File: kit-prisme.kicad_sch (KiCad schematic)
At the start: 95 parts, among them J1 Conn_01x02, J10 Conn_01x03, J11 Conn_01x04, J12 Conn_01x04, J13 Conn_01x04, J14 Conn_01x04, J15 Conn_01x04, J16 Conn_01x04, J17 Conn_01x04, J18 Conn_01x04, J19 Conn_01x04, J2 Conn_01x16, J20 Conn_01x04, J21 Conn_01x04, J22 Conn_01x04, J23 Conn_01x04, J24 Conn_01x04, J25 Conn_01x04, J26 Conn_01x04, J3 Conn_01x16, J4 Conn_01x16, J5 Conn_01x02, J6 Conn_01x02, J7 Conn_01x04, J8 Conn_01x04, J9 Conn_01x04, Q1 2N7000, Q10 2N7000, Q11 2N7000, Q2 2N7000, Q3 2N7000, Q4 2N7000, Q5 2N7000, Q6 2N7000, Q7 2N7000, Q8 2N7000, Q9 2N7000

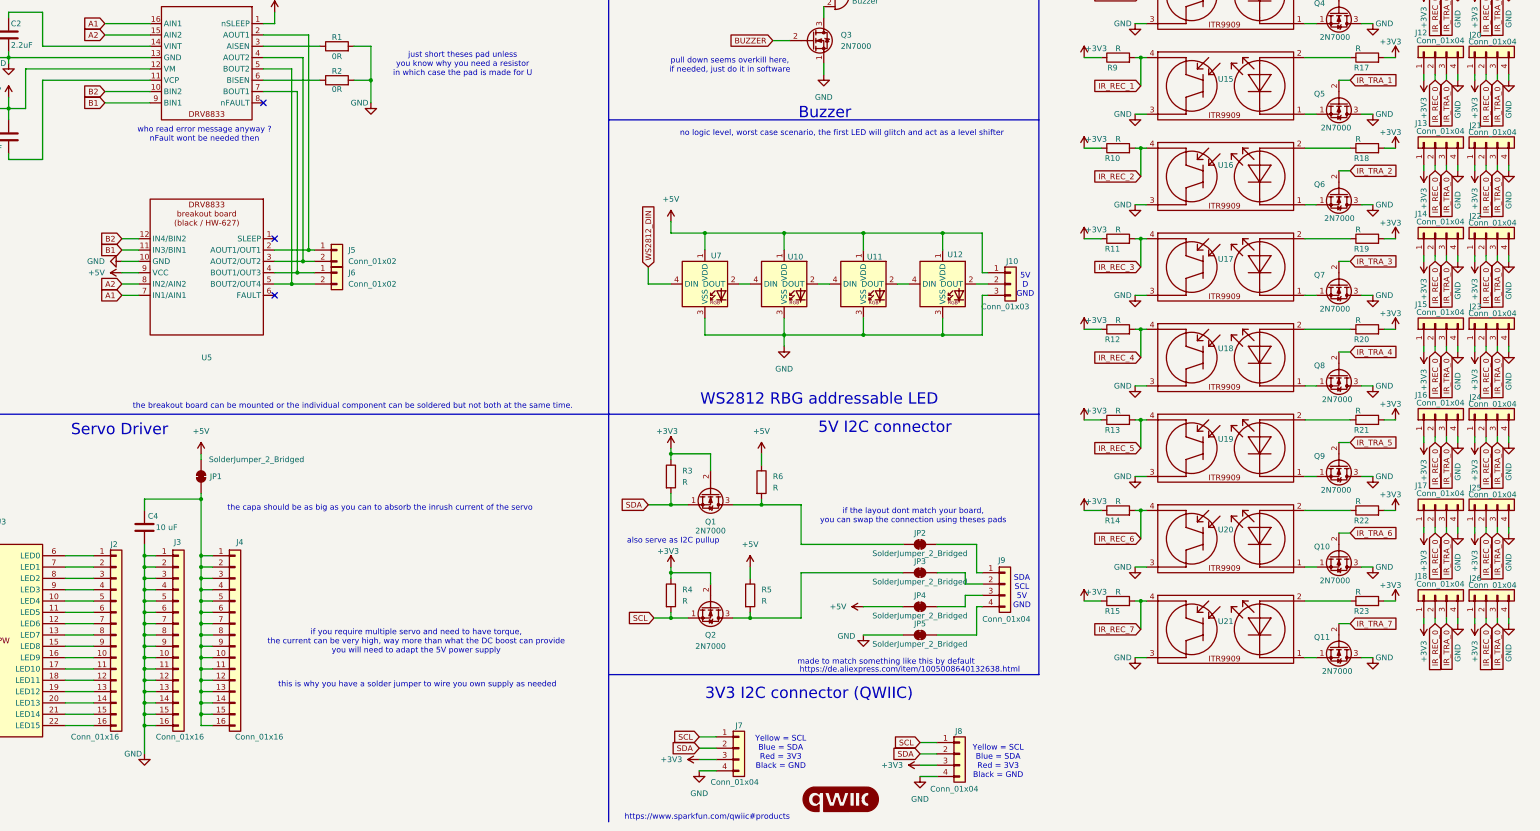
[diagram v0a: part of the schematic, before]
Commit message: looking for a good PCB layout
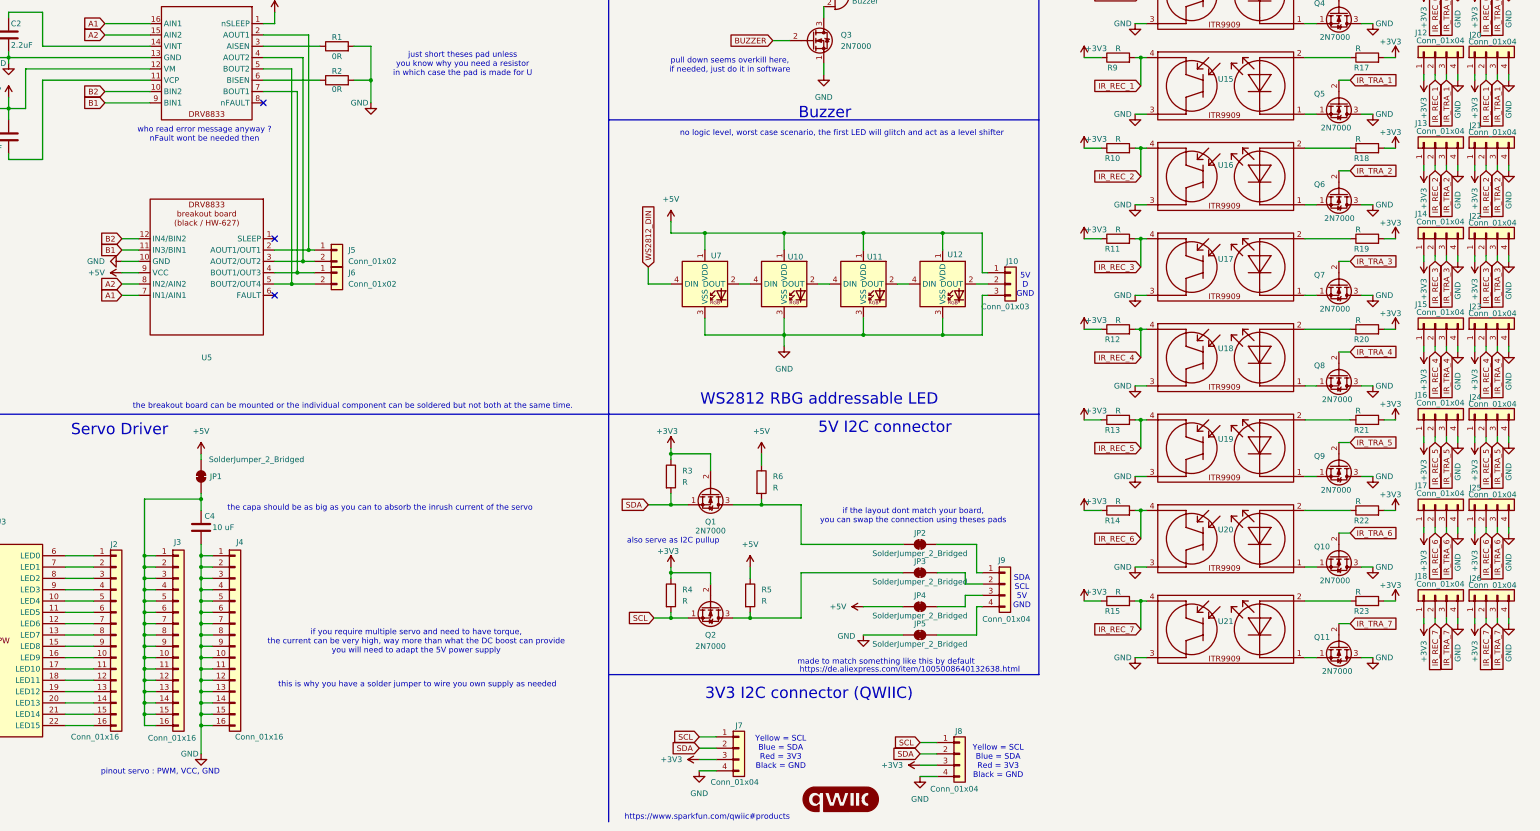
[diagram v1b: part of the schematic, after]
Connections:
- net GND: now also J4.1 (Pin_1), J4.10 (Pin_10), J4.11 (Pin_11), J4.12 (Pin_12), J4.13 (Pin_13), J4.14 (Pin_14), J4.15 (Pin_15), J4.16 (Pin_16), J4.2 (Pin_2), J4.3 (Pin_3), J4.4 (Pin_4), J4.5 (Pin_5), J4.6 (Pin_6), J4.7 (Pin_7), J4.8 (Pin_8), J4.9 (Pin_9); no longer J3.1 (Pin_1), J3.10 (Pin_10), J3.11 (Pin_11), J3.12 (Pin_12), J3.13 (Pin_13), J3.14 (Pin_14), J3.15 (Pin_15), J3.16 (Pin_16), J3.2 (Pin_2), J3.3 (Pin_3), J3.4 (Pin_4), J3.5 (Pin_5), J3.6 (Pin_6), J3.7 (Pin_7), J3.8 (Pin_8), J3.9 (Pin_9)
- net IR_REC_0: no longer J12.2 (Pin_2), J13.2 (Pin_2), J14.2 (Pin_2), J15.2 (Pin_2), J16.2 (Pin_2), J17.2 (Pin_2), J18.2 (Pin_2), J20.2 (Pin_2), J21.2 (Pin_2), J22.2 (Pin_2), J23.2 (Pin_2), J24.2 (Pin_2), J25.2 (Pin_2), J26.2 (Pin_2)
- net IR_REC_1: now also J12.2 (Pin_2), J20.2 (Pin_2)
- net IR_REC_2: now also J13.2 (Pin_2), J21.2 (Pin_2)
- net IR_REC_3: now also J14.2 (Pin_2), J22.2 (Pin_2)
- net IR_REC_4: now also J15.2 (Pin_2), J23.2 (Pin_2)
- net IR_REC_5: now also J16.2 (Pin_2), J24.2 (Pin_2)
- net IR_REC_6: now also J17.2 (Pin_2), J25.2 (Pin_2)
- net IR_REC_7: now also J18.2 (Pin_2), J26.2 (Pin_2)
- net IR_TRA_0: no longer J12.3 (Pin_3), J13.3 (Pin_3), J14.3 (Pin_3), J15.3 (Pin_3), J16.3 (Pin_3), J17.3 (Pin_3), J18.3 (Pin_3), J20.3 (Pin_3), J21.3 (Pin_3), J22.3 (Pin_3), J23.3 (Pin_3), J24.3 (Pin_3), J25.3 (Pin_3), J26.3 (Pin_3)
- net IR_TRA_1: now also J12.3 (Pin_3), J20.3 (Pin_3)
- net IR_TRA_2: now also J13.3 (Pin_3), J21.3 (Pin_3)
- net IR_TRA_3: now also J14.3 (Pin_3), J22.3 (Pin_3)
- net IR_TRA_4: now also J15.3 (Pin_3), J23.3 (Pin_3)
- net IR_TRA_5: now also J16.3 (Pin_3), J24.3 (Pin_3)
- net IR_TRA_6: now also J17.3 (Pin_3), J25.3 (Pin_3)
- net IR_TRA_7: now also J18.3 (Pin_3), J26.3 (Pin_3)
- new net: C4.1, J3.1 (Pin_1), J3.10 (Pin_10), J3.11 (Pin_11), J3.12 (Pin_12), J3.13 (Pin_13), J3.14 (Pin_14), J3.15 (Pin_15), J3.16 (Pin_16), J3.2 (Pin_2), J3.3 (Pin_3), J3.4 (Pin_4), J3.5 (Pin_5), J3.6 (Pin_6), J3.7 (Pin_7), J3.8 (Pin_8), J3.9 (Pin_9), JP1.2 (B)
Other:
- note added: "pinout servo : PWM, VCC, GND"
- moved on the sheet: C4
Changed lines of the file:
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@@
 		)
 	)
+	(text "pinout servo : PWM, VCC, GND\n"
+		(exclude_from_sim no)
+		(at 102.616 273.304 0)
+		(effects
+			(font
+				(size 1.27 1.27)
+			)
+		)
+	)
 	(text "also serve as I2C pullup"
 		(exclude_from_sim no)
@@
 	)
 	(junction
+		(at 111.76 224.79)
+		(diameter 0)
+		(color 0 0 0 0)
+	)
+	(junction
 		(at 99.06 252.73)
 		(diameter 0)
@@
 	)
 	(junction
+		(at 111.76 212.09)
+		(diameter 0)
+		(color 0 0 0 0)
+	)
+	(junction
 		(at 260.35 152.4)
 		(diameter 0)
@@
 	)
 	(junction
-		(at 111.76 212.09)
+		(at 111.76 262.89)
 		(diameter 0)
 		(color 0 0 0 0)
@@
 	)
 	(junction
-		(at 99.06 262.89)
-		(diameter 0)
-		(color 0 0 0 0)
-	)
-	(junction
 		(at 38.1 57.15)
 		(diameter 0)
@@
 	)
 	(junction
-		(at 111.76 224.79)
-		(diameter 0)
-		(color 0 0 0 0)
-	)
-	(junction
 		(at 99.06 242.57)
 		(diameter 0)
@@
 	(wire
 		(pts
+			(xy 111.76 222.25) (xy 111.76 224.79)
+		)
+		(stroke
+			(width 0)
+			(type default)
+		)
+	)
+	(wire
+		(pts
 			(xy 242.57 171.45) (xy 242.57 175.26)
 		)
@@
 	(wire
 		(pts
-			(xy 99.06 222.25) (xy 99.06 224.79)
-		)
-		(stroke
-			(width 0)
-			(type default)
-		)
-	)
-	(wire
-		(pts
 			(xy 278.13 175.26) (xy 287.02 175.26)
 		)
@@
 	(wire
 		(pts
-			(xy 111.76 212.09) (xy 111.76 224.79)
-		)
-		(stroke
-			(width 0)
-			(type default)
-		)
-	)
-	(wire
-		(pts
 			(xy 322.58 133.35) (xy 322.58 139.7)
 		)
@@
 	(wire
 		(pts
+			(xy 111.76 212.09) (xy 111.76 214.63)
+		)
+		(stroke
+			(width 0)
+			(type default)
+		)
+	)
+	(wire
+		(pts
 			(xy 241.3 25.4) (xy 243.84 25.4)
 		)
@@
 	(wire
 		(pts
-			(xy 99.06 214.63) (xy 99.06 212.09)
+			(xy 99.06 212.09) (xy 99.06 224.79)
 		)
 		(stroke
@@
 	(wire
 		(pts
+			(xy 111.76 262.89) (xy 111.76 269.24)
+		)
+		(stroke
+			(width 0)
+			(type default)
+		)
+	)
+	(wire
+		(pts
 			(xy 326.39 62.23) (xy 326.39 63.5)
 		)
@@
 	(wire
 		(pts
-			(xy 99.06 262.89) (xy 99.06 269.24)
-		)
-		(stroke
-			(width 0)
-			(type default)
-		)
-	)
-	(wire
-		(pts
 			(xy 45.72 252.73) (xy 43.18 252.73)
 		)
@@
 		)
 	)
-	(global_label "IR_REC_0"
+	(global_label "IR_REC_1"
 		(shape input)
 		(at 400.05 118.11 270)
@@
 		)
 	)
-	(global_label "IR_REC_0"
+	(global_label "IR_REC_1"
 		(shape input)
 		(at 388.62 118.11 270)
@@
 		)
 	)
-	(global_label "IR_TRA_0"
+	(global_label "IR_TRA_5"
 		(shape input)
 		(at 402.59 199.39 270)
@@
 		)
 	)
-	(global_label "IR_TRA_0"
+	(global_label "IR_TRA_7"
 		(shape input)
 		(at 391.16 240.03 270)
@@
 		)
 	)
-	(global_label "IR_REC_0"
+	(global_label "IR_REC_6"
 		(shape input)
 		(at 388.62 219.71 270)
@@
 		)
 	)
-	(global_label "IR_TRA_0"
+	(global_label "IR_TRA_1"
 		(shape input)
 		(at 402.59 118.11 270)
@@
 		)
 	)
-	(global_label "IR_REC_0"
+	(global_label "IR_REC_7"
 		(shape input)
 		(at 400.05 240.03 270)
@@
 		)
 	)
-	(global_label "IR_TRA_0"
+	(global_label "IR_TRA_3"
 		(shape input)
 		(at 402.59 158.75 270)
@@
 		)
 	)
-	(global_label "IR_TRA_0"
+	(global_label "IR_TRA_4"
 		(shape input)
 		(at 391.16 179.07 270)
@@
 		)
 	)
-	(global_label "IR_REC_0"
+	(global_label "IR_REC_4"
 		(shape input)
 		(at 388.62 179.07 270)
@@
 		)
 	)
-	(global_label "IR_TRA_0"
+	(global_label "IR_TRA_6"
 		(shape input)
 		(at 402.59 219.71 270)
@@
 		)
 	)
-	(global_label "IR_TRA_0"
+	(global_label "IR_TRA_2"
 		(shape input)
 		(at 391.16 138.43 270)
@@
 		)
 	)
-	(global_label "IR_TRA_0"
+	(global_label "IR_TRA_3"
 		(shape input)
 		(at 391.16 158.75 270)
@@
 		)
 	)
-	(global_label "IR_REC_0"
+	(global_label "IR_REC_2"
 		(shape input)
 		(at 400.05 138.43 270)
@@
 		)
 	)
-	(global_label "IR_TRA_0"
+	(global_label "IR_TRA_2"
 		(shape input)
 		(at 402.59 138.43 270)
@@
 		)
 	)
-	(global_label "IR_REC_0"
+	(global_label "IR_REC_4"
 		(shape input)
 		(at 400.05 179.07 270)
@@
 		)
 	)
-	(global_label "IR_REC_0"
+	(global_label "IR_REC_5"
 		(shape input)
 		(at 400.05 199.39 270)
@@
 		)
 	)
-	(global_label "IR_TRA_0"
+	(global_label "IR_TRA_5"
 		(shape input)
 		(at 391.16 199.39 270)
@@
 		)
 	)
-	(global_label "IR_REC_0"
+	(global_label "IR_REC_3"
 		(shape input)
 		(at 388.62 158.75 270)
@@
 		)
 	)
-	(global_label "IR_REC_0"
+	(global_label "IR_REC_2"
 		(shape input)
 		(at 388.62 138.43 270)
@@
 		)
 	)
-	(global_label "IR_REC_0"
+	(global_label "IR_REC_5"
 		(shape input)
 		(at 388.62 199.39 270)
@@
 		)
 	)
-	(global_label "IR_REC_0"
+	(global_label "IR_REC_6"
 		(shape input)
 		(at 400.05 219.71 270)
@@
 		)
 	)
-	(global_label "IR_TRA_0"
+	(global_label "IR_TRA_1"
 		(shape input)
 		(at 391.16 118.11 270)
@@
 		)
 	)
-	(global_label "IR_TRA_0"
+	(global_label "IR_TRA_7"
 		(shape input)
 		(at 402.59 240.03 270)
@@
 		)
 	)
-	(global_label "IR_REC_0"
+	(global_label "IR_REC_7"
 		(shape input)
 		(at 388.62 240.03 270)
@@
 		)
 	)
-	(global_label "IR_TRA_0"
+	(global_label "IR_TRA_6"
 		(shape input)
 		(at 391.16 219.71 270)
@@
 		)
 	)
-	(global_label "IR_TRA_0"
+	(global_label "IR_TRA_4"
 		(shape input)
 		(at 402.59 179.07 270)
@@
 		)
 	)
-	(global_label "IR_REC_0"
+	(global_label "IR_REC_3"
 		(shape input)
 		(at 400.05 158.75 270)
@@
 	(symbol
 		(lib_id "power:GND")
-		(at 99.06 269.24 0)
+		(at 111.76 269.24 0)
 		(unit 1)
 		(exclude_from_sim no)
@@
 		(dnp no)
 		(property "Reference" "#PWR013"
-			(at 99.06 275.59 0)
+			(at 111.76 275.59 0)
 			(effects
 				(font
@@
 		)
 		(property "Value" "GND"
-			(at 96.52 269.24 0)
+			(at 109.22 269.24 0)
 			(effects
 				(font
@@
 		)
 		(property "Footprint" ""
-			(at 99.06 269.24 0)
+			(at 111.76 269.24 0)
 			(effects
 				(font
@@
 		)
 		(property "Datasheet" ""
-			(at 99.06 269.24 0)
+			(at 111.76 269.24 0)
 			(effects
 				(font
@@
 		)
 		(property "Description" "Power symbol creates a global label with name \"GND\" , ground"
-			(at 99.06 269.24 0)
+			(at 111.76 269.24 0)
 			(effects
 				(font
@@
 		)
 		(property "Value" "Conn_01x16"
-			(at 101.6 265.43 0)
+			(at 99.822 265.684 0)
 			(effects
 				(font
@@
 	(symbol
 		(lib_id "Device:C")
-		(at 99.06 218.44 0)
+		(at 111.76 218.44 0)
 		(unit 1)
 		(exclude_from_sim no)
@@
 		(dnp no)
 		(property "Reference" "C4"
-			(at 99.822 215.9 0)
+			(at 112.522 215.9 0)
 			(effects
 				(font
@@
 		)
 		(property "Value" "10 uF"
-			(at 101.6 218.44 0)
+			(at 114.3 218.44 0)
 			(effects
 				(font
@@
 		)
 		(property "Footprint" "Capacitor_SMD:C_0805_2012Metric_Pad1.18x1.45mm_HandSolder"
-			(at 100.0252 222.25 0)
+			(at 112.7252 222.25 0)
 			(effects
 				(font
@@
 		)
 		(property "Datasheet" "~"
-			(at 99.06 218.44 0)
+			(at 111.76 218.44 0)
 			(effects
 				(font
@@
 		)
 		(property "Description" "Unpolarized capacitor"
-			(at 99.06 218.44 0)
+			(at 111.76 218.44 0)
 			(effects
 				(font
